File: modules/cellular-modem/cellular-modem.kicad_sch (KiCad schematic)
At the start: 23 parts, among them J1 MM60-mini-PCIe, J2 MM60-EZH059-B5-R650, U1 TXV0108RGYR, U2 TXV0108RGYR, U3 TXV0108RGYR, U4 TPS631000DRLR, U5 TPS631000DRLR

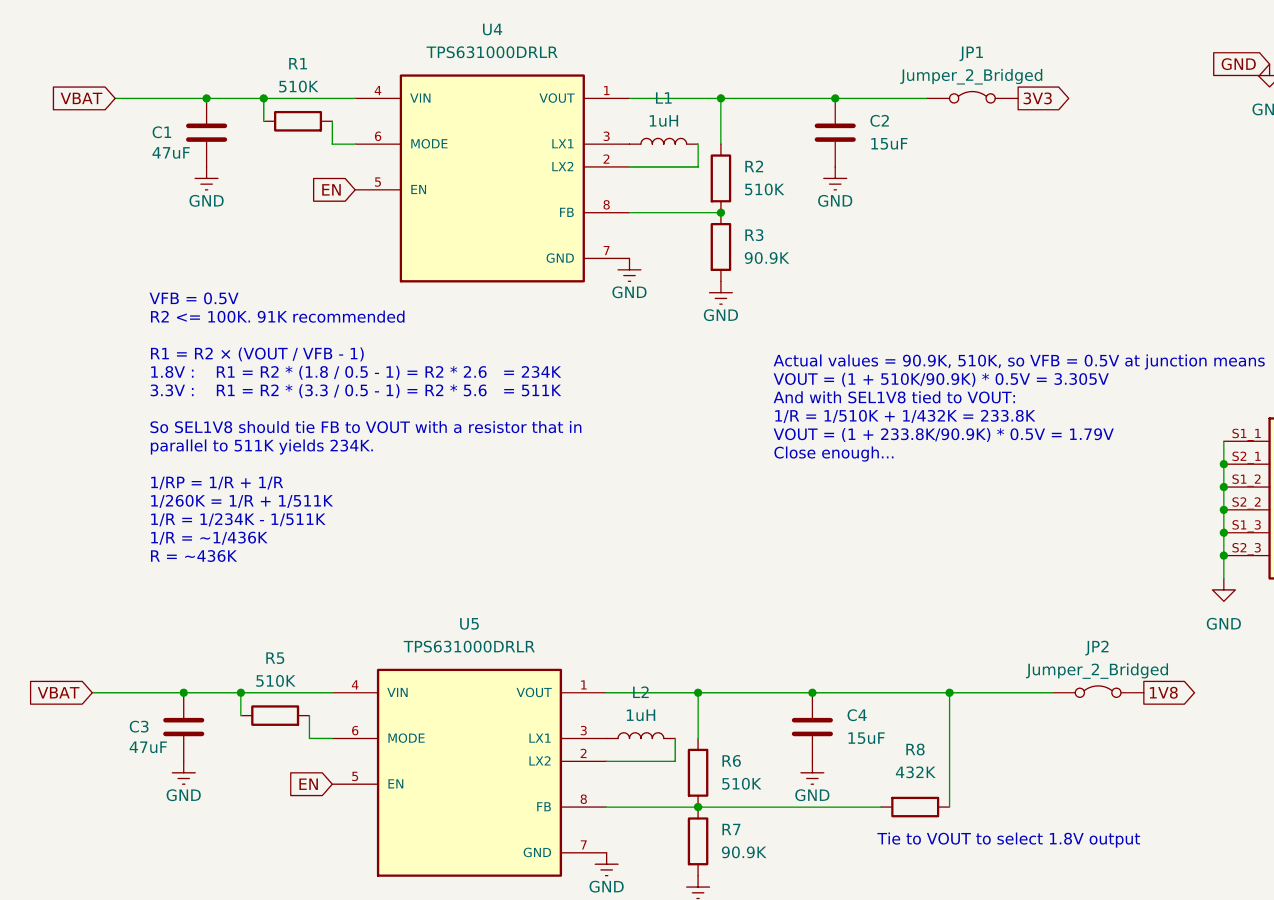
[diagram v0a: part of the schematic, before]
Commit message: Updating all modules
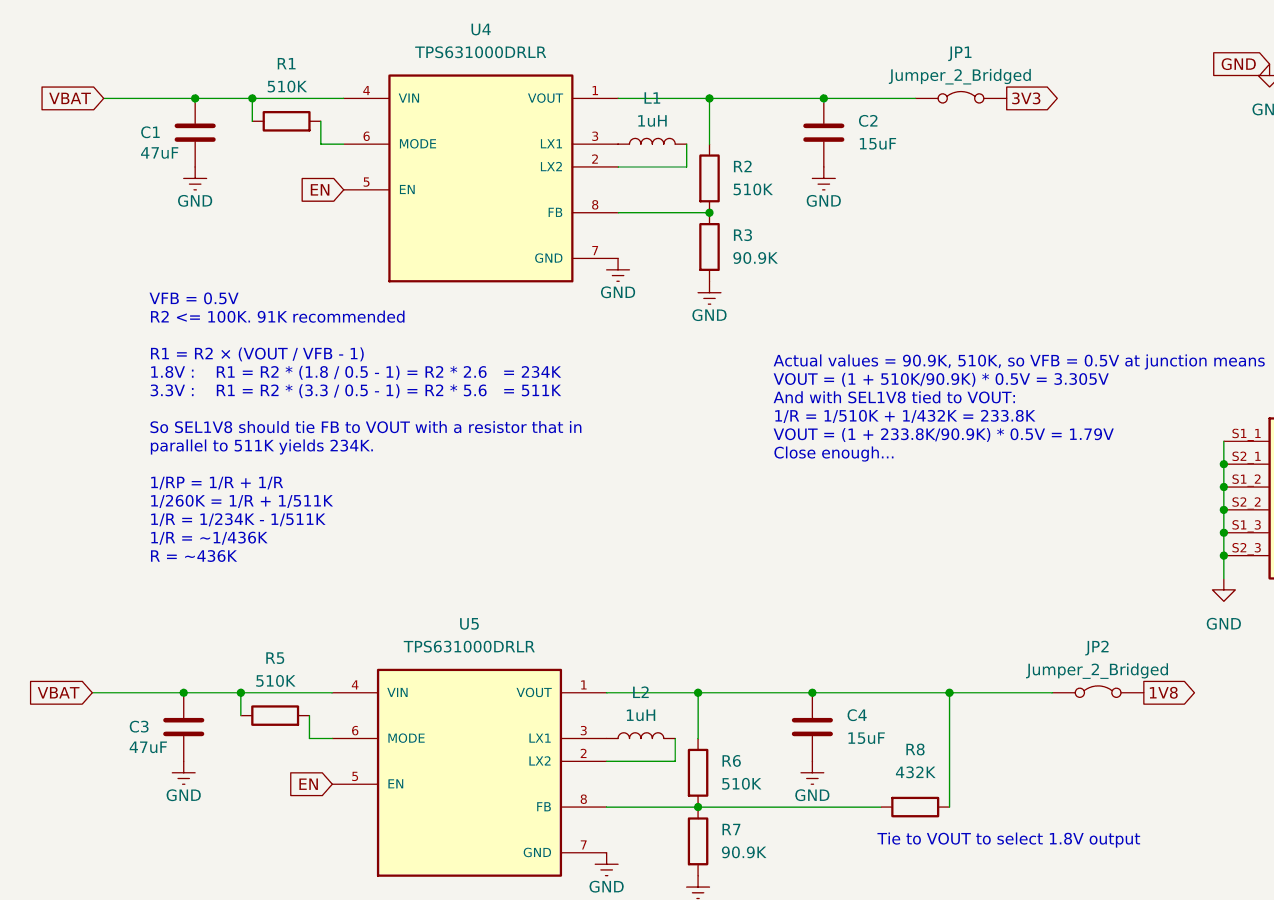
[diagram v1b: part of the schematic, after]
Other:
- moved on the sheet: C1, C2, JP1, L1, R1, R2, R3, U4
